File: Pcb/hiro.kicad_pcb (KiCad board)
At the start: 2 copper layers, 80.1 x 107.1 mm, 15 parts, among them J1 Micro_SD_Card_Det_Hirose_DM3AT, J2 AudioJack3, J3 Conn_01x08, SW1 RotaryEncoder_Switch, U1 XIAO-ESP32-S3-Plus-SMD, U2 PCM5102A, U3 MAX98357A

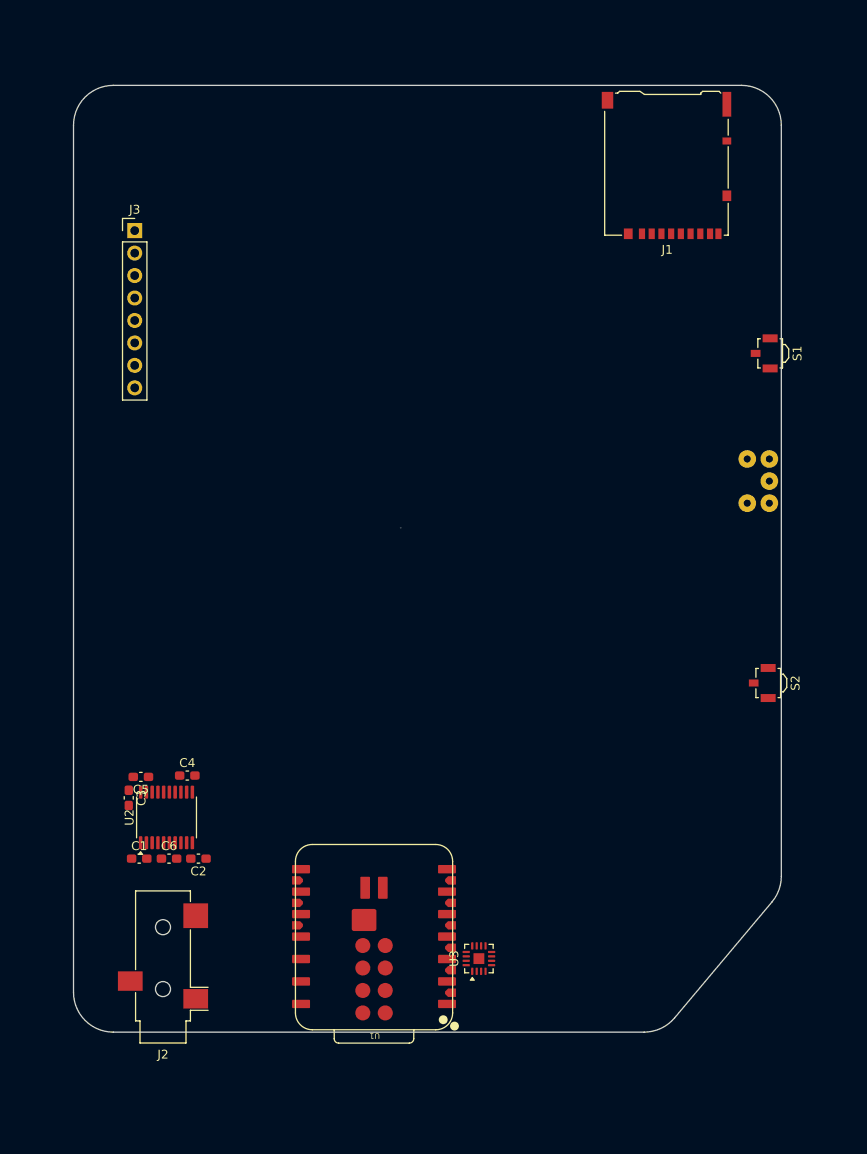
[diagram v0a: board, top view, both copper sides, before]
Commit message: Some stuffs
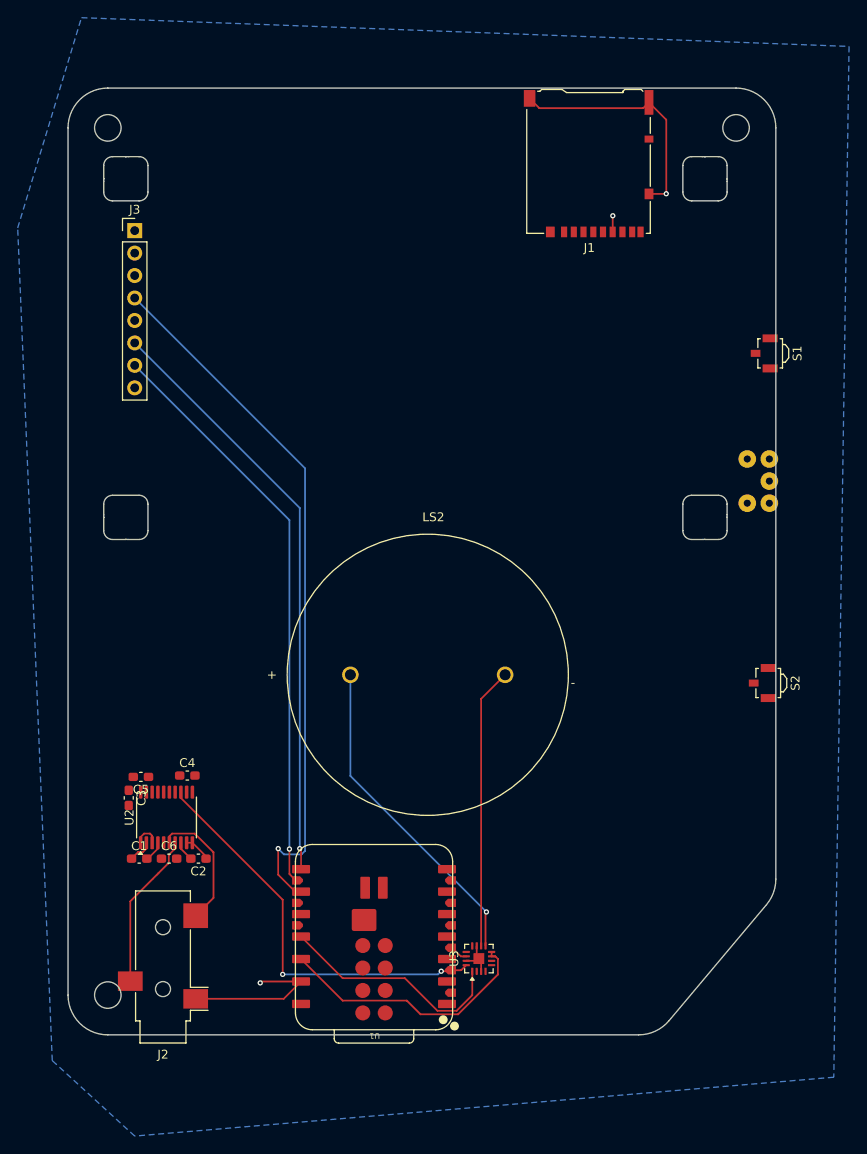
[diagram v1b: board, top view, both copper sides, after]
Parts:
- added LS2: CVS-3108, Spkr:CUI_CVS-3108, F.Cu at (91.8, 100.2)
- moved J1 8.81 mm to (110.0, 42.4)
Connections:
- J1 pad 2: /CS -> /CS1
- U1 pad 23: unconnected-(U1-GPIO13_DVP_PCLK_SPI_SCK1-Pad23) -> /CS1
- U3 pad 17: unconnected-(U3-PAD-Pad17) -> GND
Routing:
- net /SCK: track 0.00 -> 80.3 mm, vias 0 -> 1
- net /DC: track 0.00 -> 67.3 mm, vias 0 -> 1
- net /MOSI: track 0.00 -> 66.0 mm, vias 0 -> 1
- net GND: track 0.00 -> 57.3 mm, vias 0 -> 3
- net /BCK: track 0.00 -> 46.6 mm, vias 0 -> 2
- net Net-(U3-OUTP): track 0.00 -> 37.1 mm, vias 0 -> 1
- net Net-(U3-OUTN): track 0.00 -> 31.8 mm
- net +3.3V: track 0.00 -> 29.8 mm
- net /DIN1: track 0.00 -> 26.3 mm
- net Net-(U2-OUTR): track 0.00 -> 17.8 mm
- net Net-(U2-OUTL): track 0.00 -> 14.7 mm
- net Net-(U2-CAPP): track 0.00 -> 2.81 mm
- net Net-(U2-CAPM): track 0.00 -> 2.38 mm
- net Net-(U2-AVDD): track 0.00 -> 2.26 mm
- net /LCK: track 0.00 -> 2.17 mm
- added copper zone on B.Cu, net GND
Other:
- outline, holes or cut-outs redrawn
